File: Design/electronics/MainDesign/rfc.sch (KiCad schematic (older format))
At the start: 24 parts, among them IC1 L298, IC2 L298, J1 CONN_02X20, J2 CONN_01X03, J3 CONN_01X03, M1 Motor, M2 Motor, M3 Motor, M4 Motor, U1 HC-SR04, U2 HC-SR04, U3 HC-SR04, U4 HC-SR04

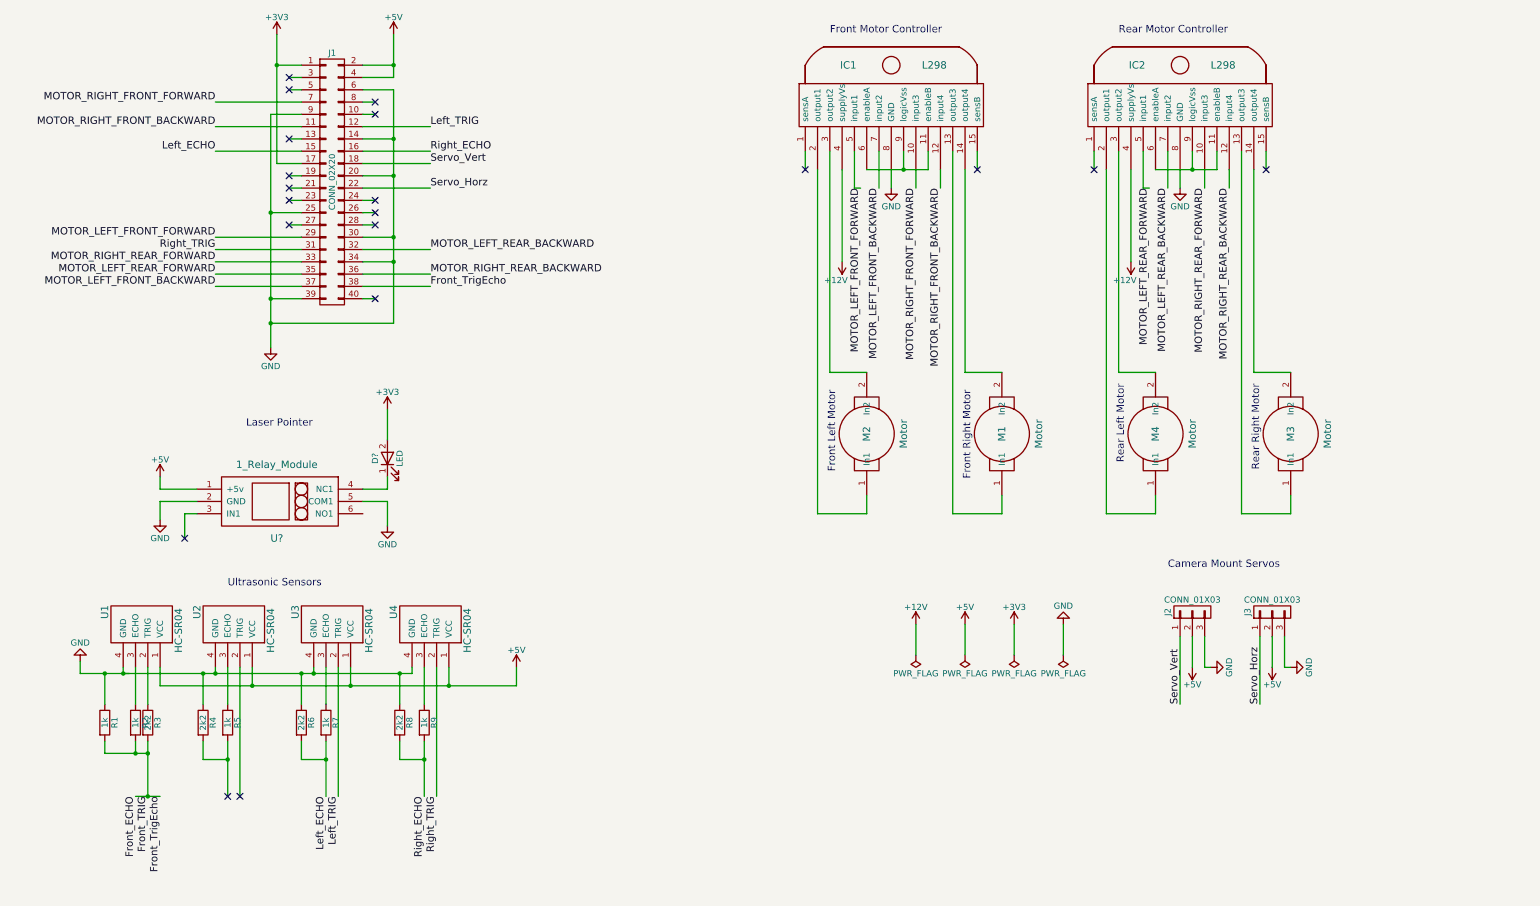
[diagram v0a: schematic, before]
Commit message: Duck shoot changes to electronics design
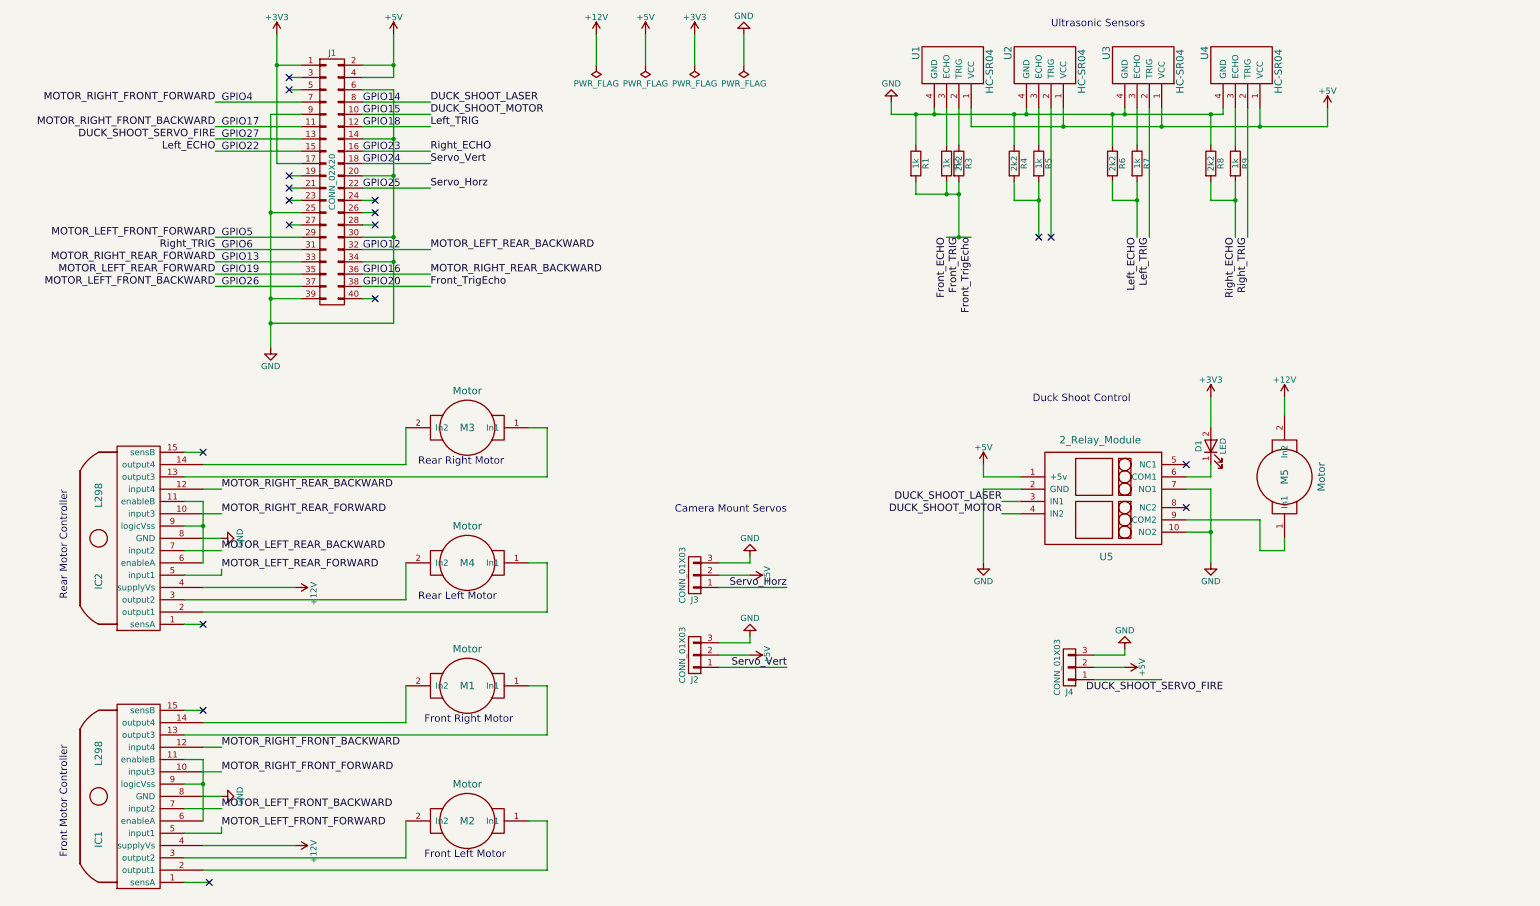
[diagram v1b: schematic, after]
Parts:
- removed U?: 1_Relay_Module, symbol 1_Relay_Module
- added J4: CONN_01X03, symbol CONN_01X03
- added M5: Motor, symbol Motor
- added U5: 2_Relay_Module, symbol 2_Relay_Module
- gave numbers to parts that had none: 1
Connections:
- net +12V: now also M5.2 (In2)
- net +5V: now also J4.2 (P2), U5.1 (+5v)
- net GND: now also J4.3 (P3), U5.10 (NO2), U5.2 (GND), U5.7 (NO1)
- net DUCK_SHOOT_MOTOR: now reaches J1.10 (P10)
- net DUCK_SHOOT_MOTOR: now also U5.4 (IN2)
- net DUCK_SHOOT_SERVO_FIRE: now reaches J1.13 (P13)
- net DUCK_SHOOT_LASER: now reaches J1.8 (P8)
- net DUCK_SHOOT_LASER: now also U5.3 (IN1)
- net at D1.1 (K): now also U5.6 (COM1)
- new net: M5.1 (In1), U5.9 (COM2)
- no-connect marks 20 -> 18
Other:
- note added: "Duck Shoot Control"
- note added: "GPIO12"
- note added: "GPIO13"
- note added: "GPIO14"
- note added: "GPIO15"
- note added: "GPIO16"
- note added: "GPIO17"
- note added: "GPIO18"
- note added: "GPIO19"
- note added: "GPIO20"
- note added: "GPIO22"
- note added: "GPIO23"
- note added: "GPIO24"
- note added: "GPIO25"
- note added: "GPIO26"
- note added: "GPIO27"
- note added: "GPIO4"
- note added: "GPIO5"
- note added: "GPIO6"
- note removed: "Laser Pointer"
- moved on the sheet: D1, IC1, IC2, J2, J3, M1, M2, M3, M4, R1, R2, R3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
